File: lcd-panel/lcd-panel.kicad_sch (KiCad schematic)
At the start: 42 parts, among them J1 USB wire, J2 LCD FPC connector, J3 Fan Socket, Q1 AO3400A, Q2 AO3401A, Q3 AO3400A, U1 FT232HL-REEL, U2 93LC56BT-I/OT, U3 USBLC6-2SC6, Y1 12 MHz, 20 pF load

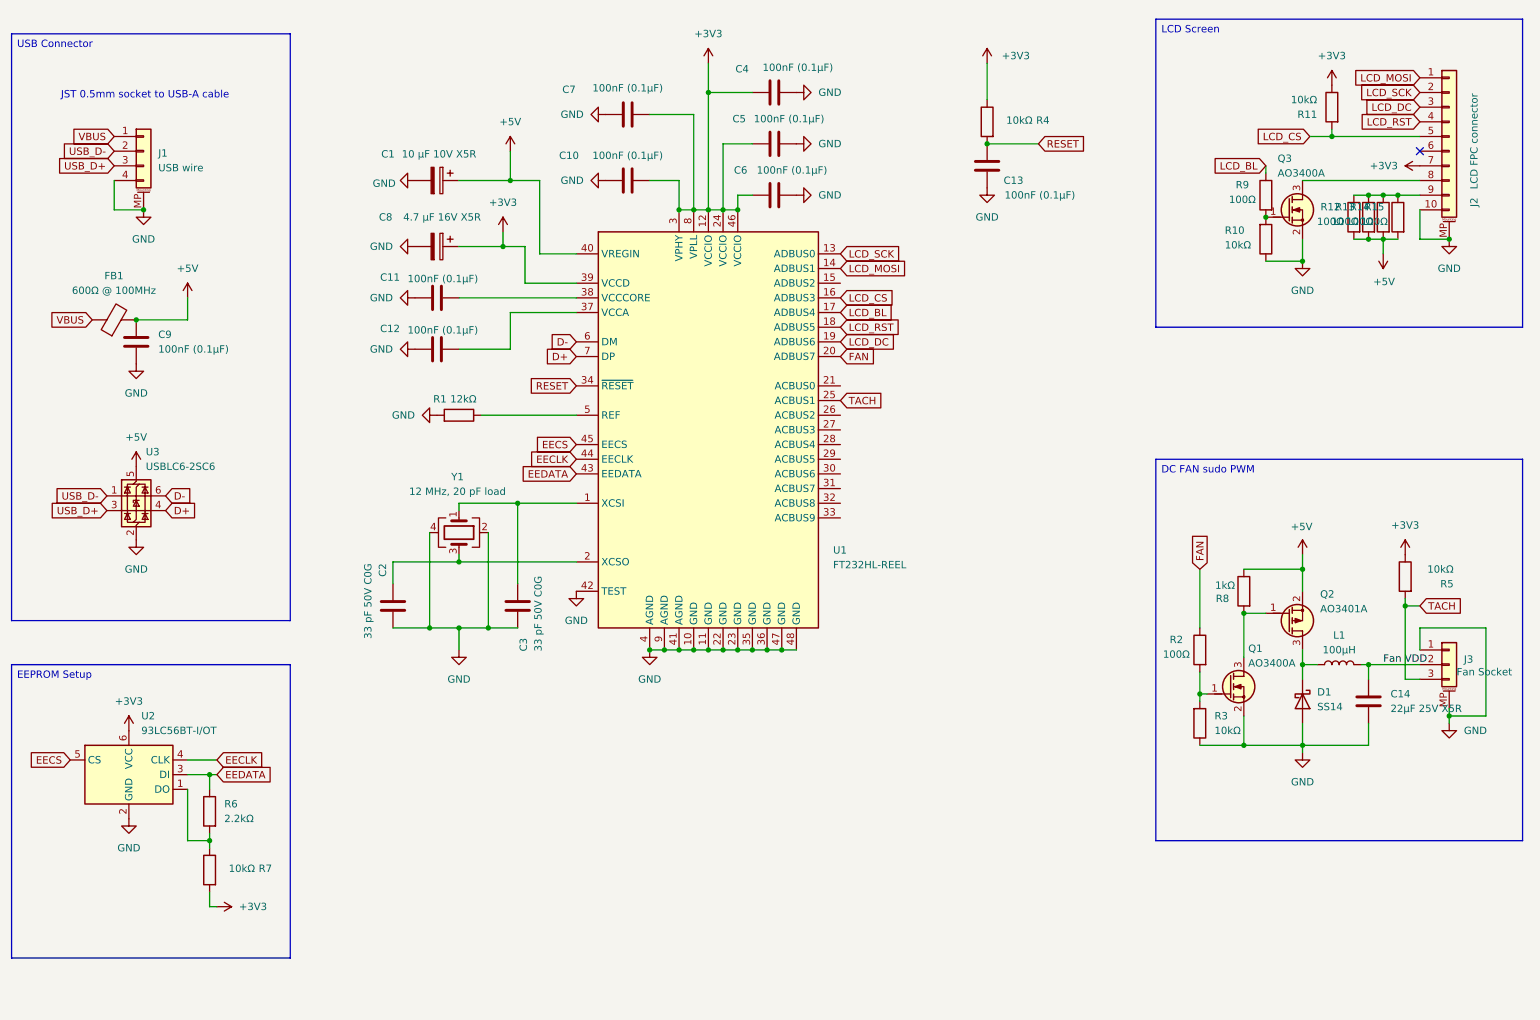
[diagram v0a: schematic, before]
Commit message: Reworking the rest of the schematics
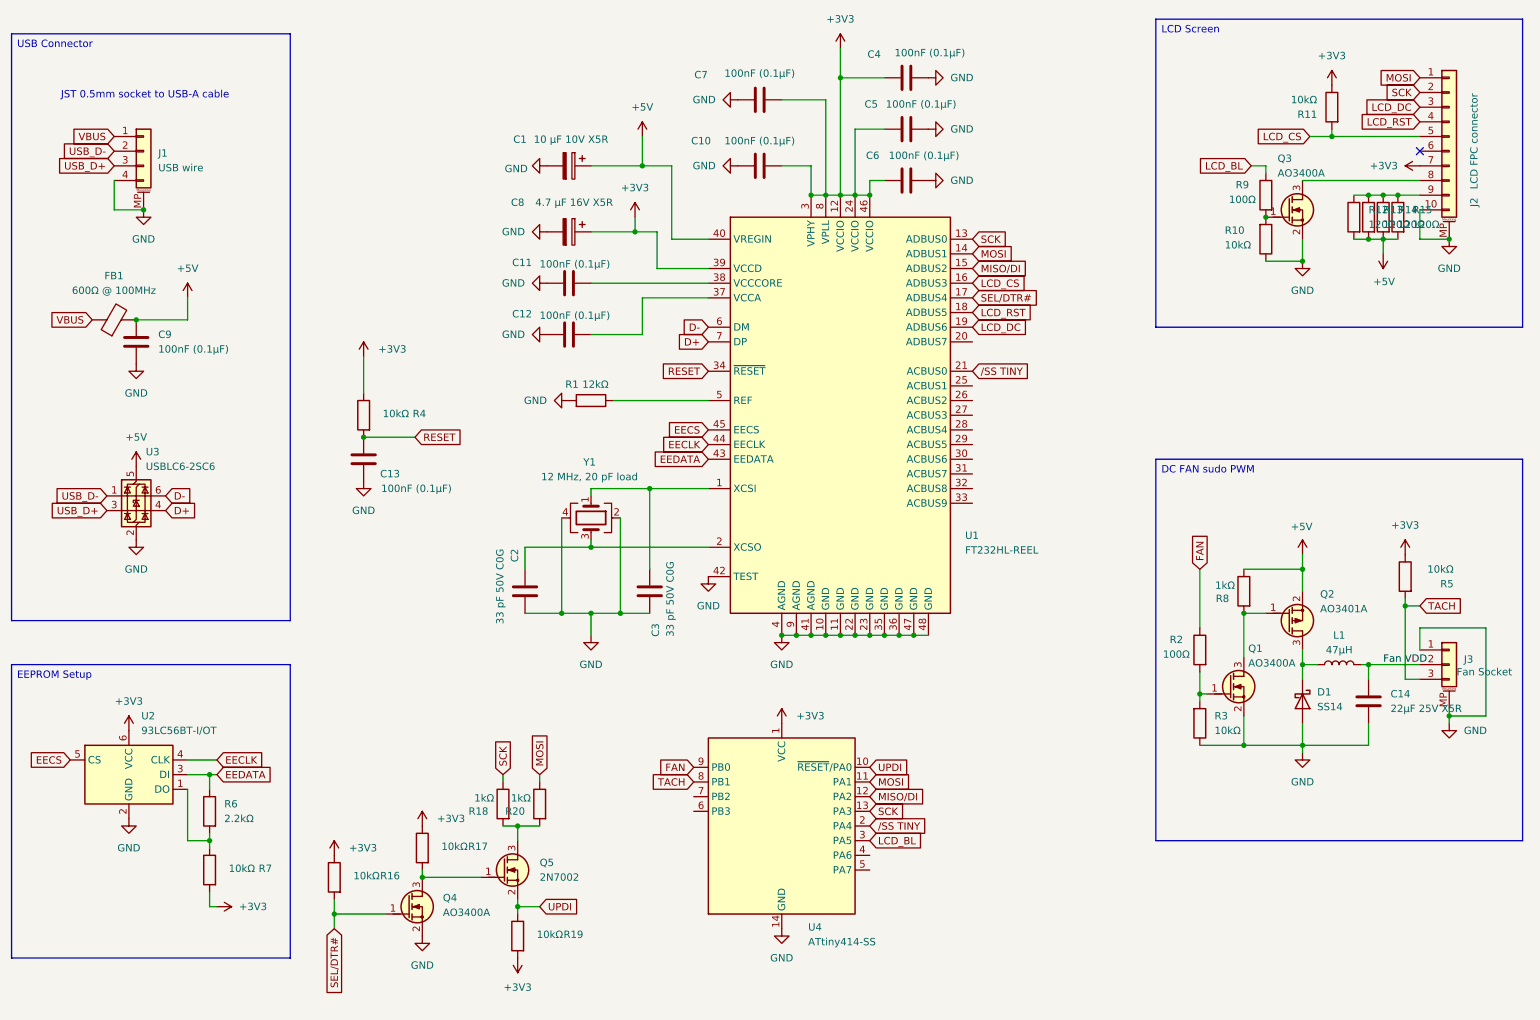
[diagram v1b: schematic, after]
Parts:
- added Q4: AO3400A, PCM_Package_TO_SOT_SMD_AKL:SOT-23, symbol PCM_Transistor_MOSFET_AKL:AO3400A
- added Q5: 2N7002, PCM_Package_TO_SOT_SMD_AKL:SOT-23, symbol PCM_Transistor_MOSFET_AKL:2N7002
- added R16, R17, R19: 10kΩ, Resistor_SMD:R_0402_1005Metric, symbol PCM_Resistor_AKL:R_0603
- added R18, R20: 1kΩ, Resistor_SMD:R_0402_1005Metric, symbol PCM_Resistor_AKL:R_0603
- added U4: ATtiny414-SS, Package_SO:SOIC-14_3.9x8.7mm_P1.27mm, symbol MCU_Microchip_ATtiny:ATtiny414-SS
- L1: value 100µH -> 47µH
- R12, R13, R14, R15: value 100Ω -> 120Ω; LCSC C22775 -> C22787
- R2, R9: footprint Resistor_SMD:R_0603_1608Metric -> Resistor_SMD:R_0402_1005Metric; LCSC C22775 -> C25076
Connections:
- net +3V3: now also R16.2, R17.2, R19.1, U4.1 (VCC)
- net FAN: now also U4.9 (PB0); no longer U1.20 (ADBUS7)
- net GND: now also Q4.2 (S), U4.14 (GND)
- net LCD_BL: now also U4.3 (PA5); no longer U1.17 (ADBUS4)
- net TACH: now also U4.8 (PB1); no longer U1.25 (ACBUS1)
- net MISO/DI: now reaches U1.15 (ADBUS2)
- net MISO/DI: now also U4.12 (PA2)
- net /SS TINY: now reaches U1.21 (ACBUS0)
- net /SS TINY: now also U4.2 (PA4)
- net LCD_MOSI renamed MOSI
- net MOSI: now also R20.2, U4.11 (PA1)
- net LCD_SCK renamed SCK
- net SCK: now also R18.2, U4.13 (PA3)
- new net: Q5.3 (D), R18.1, R20.1
- new net: Q4.3 (D), Q5.1 (G), R17.1
- new net SEL/DTR#: Q4.1 (G), R16.1, U1.17 (ADBUS4)
- new net UPDI: Q5.2 (S), R19.2, U4.10 (~{RESET}/PA0)
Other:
- moved on the sheet: C1, C10, C11, C12, C13, C2, C3, C4, C5, C6, C7, C8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
